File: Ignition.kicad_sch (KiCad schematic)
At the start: 12 parts, among them Q1 AOI21357, Q2 2N7002, Q3 2N7002, Q5 AOI21357

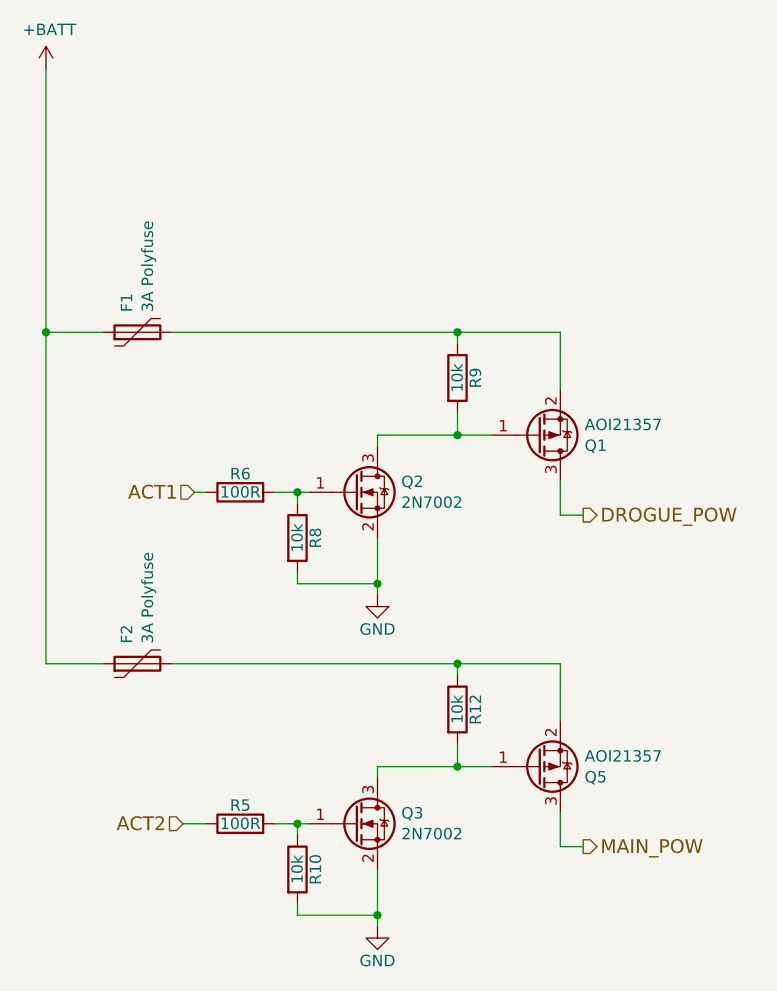
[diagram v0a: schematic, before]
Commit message: fix mosfet
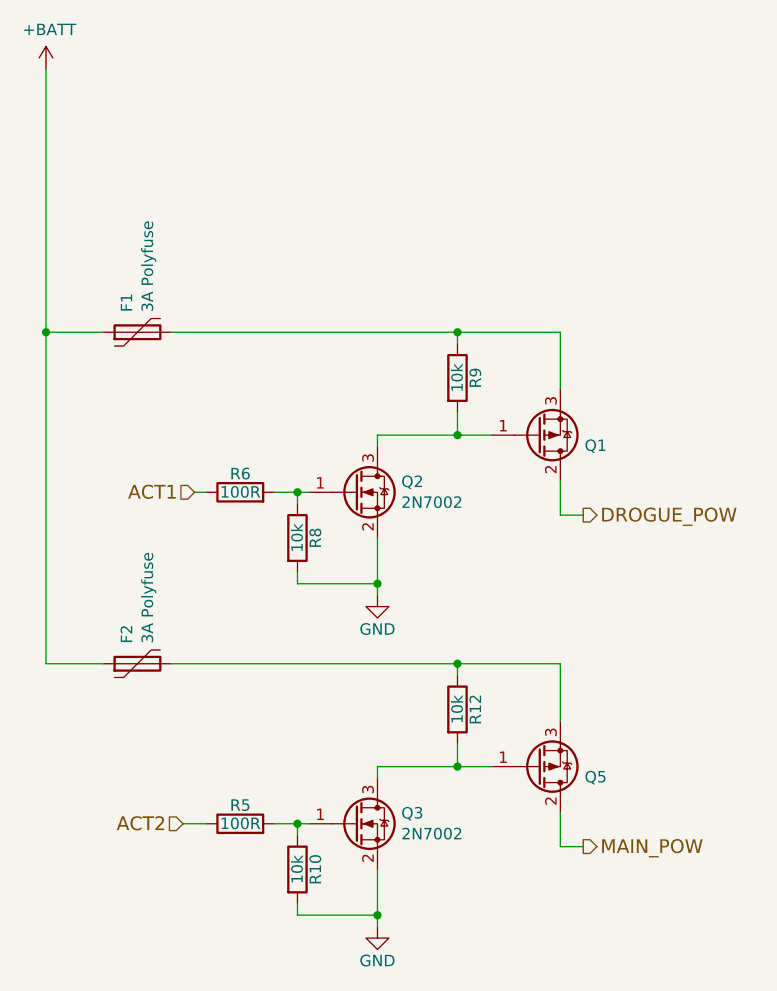
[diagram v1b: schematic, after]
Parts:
- Q1, Q5: value AOI21357 -> (none); footprint Package_TO_SOT_THT:TO-251-3_Vertical -> (none); symbol Device:Q_PMOS_GSD -> Device:Q_PMOS_GDS
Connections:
- net DROGUE_POW: now also Q1.2 (D); no longer Q1.3 (D)
- net MAIN_POW: now also Q5.2 (D); no longer Q5.3 (D)
- net at F1.2, R9.1: now also Q1.3 (S); no longer Q1.2 (S)
- net at F2.2, R12.1: now also Q5.3 (S); no longer Q5.2 (S)
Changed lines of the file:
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@@
+    (stroke (width 0) (type default) (color 0 0 0 0))
+  )
+  (wire (pts (xy 139.7 63.5) (xy 139.7 66.04))
+    (stroke (width 0) (type default) (color 0 0 0 0))
+  )
+  (wire (pts (xy 121.92 110.49) (xy 121.92 109.22))
+    (stroke (width 0) (type default) (color 0 0 0 0))
+  )
+  (wire (pts (xy 130.81 82.55) (xy 130.81 83.82))
+    (stroke (width 0) (type default) (color 0 0 0 0))
+  )
+  (wire (pts (xy 121.92 119.38) (xy 130.81 119.38))
+    (stroke (width 0) (type default) (color 0 0 0 0))
+  )
+  (wire (pts (xy 109.22 109.22) (xy 111.76 109.22))
+    (stroke (width 0) (type default) (color 0 0 0 0))
+  )
+  (wire (pts (xy 139.7 66.04) (xy 143.51 66.04))
+    (stroke (width 0) (type default) (color 0 0 0 0))
+  )
+  (wire (pts (xy 119.38 109.22) (xy 121.92 109.22))
+    (stroke (width 0) (type default) (color 0 0 0 0))
+  )
+  (wire (pts (xy 130.81 66.04) (xy 130.81 67.31))
+    (stroke (width 0) (type default) (color 0 0 0 0))
+  )
+  (wire (pts (xy 139.7 92.71) (xy 139.7 91.44))
+    (stroke (width 0) (type default) (color 0 0 0 0))
+  )
+  (wire (pts (xy 139.7 102.87) (xy 143.51 102.87))
+    (stroke (width 0) (type default) (color 0 0 0 0))
+  )
+  (wire (pts (xy 121.92 81.28) (xy 121.92 82.55))
     (stroke (width 0) (type default) (color 0 0 0 0))
   )
@@
     (stroke (width 0) (type default) (color 0 0 0 0))
   )
-  (wire (pts (xy 139.7 63.5) (xy 139.7 66.04))
-    (stroke (width 0) (type default) (color 0 0 0 0))
-  )
-  (wire (pts (xy 121.92 110.49) (xy 121.92 109.22))
-    (stroke (width 0) (type default) (color 0 0 0 0))
-  )
-  (wire (pts (xy 130.81 82.55) (xy 130.81 83.82))
-    (stroke (width 0) (type default) (color 0 0 0 0))
-  )
-  (wire (pts (xy 121.92 119.38) (xy 130.81 119.38))
-    (stroke (width 0) (type default) (color 0 0 0 0))
-  )
-  (wire (pts (xy 109.22 109.22) (xy 111.76 109.22))
-    (stroke (width 0) (type default) (color 0 0 0 0))
-  )
-  (wire (pts (xy 139.7 66.04) (xy 143.51 66.04))
-    (stroke (width 0) (type default) (color 0 0 0 0))
-  )
-  (wire (pts (xy 119.38 109.22) (xy 121.92 109.22))
-    (stroke (width 0) (type default) (color 0 0 0 0))
-  )
-  (wire (pts (xy 130.81 66.04) (xy 130.81 67.31))
-    (stroke (width 0) (type default) (color 0 0 0 0))
-  )
-  (wire (pts (xy 139.7 92.71) (xy 139.7 91.44))
-    (stroke (width 0) (type default) (color 0 0 0 0))
-  )
-  (wire (pts (xy 139.7 102.87) (xy 143.51 102.87))
-    (stroke (width 0) (type default) (color 0 0 0 0))
-  )
-  (wire (pts (xy 121.92 81.28) (xy 121.92 82.55))
-    (stroke (width 0) (type default) (color 0 0 0 0))
-  )
   (wire (pts (xy 93.98 54.61) (xy 100.33 54.61))
     (stroke (width 0) (type default) (color 0 0 0 0))
@@
     (stroke (width 0) (type default) (color 0 0 0 0))
   )
-  (wire (pts (xy 151.13 74.93) (xy 151.13 71.12))
-    (stroke (width 0) (type default) (color 0 0 0 0))
-  )
   (wire (pts (xy 130.81 102.87) (xy 130.81 104.14))
     (stroke (width 0) (type default) (color 0 0 0 0))
@@
   )
   (wire (pts (xy 130.81 66.04) (xy 139.7 66.04))
+    (stroke (width 0) (type default) (color 0 0 0 0))
+  )
+  (wire (pts (xy 151.13 71.12) (xy 151.13 74.93))
     (stroke (width 0) (type default) (color 0 0 0 0))
   )
@@
     (pin "2")
   )
-  (symbol (lib_id "Device:Q_PMOS_GSD") (at 148.59 102.87 0) (mirror x) (unit 1)
+  (symbol (lib_id "Device:Q_PMOS_GDS") (at 148.59 102.87 0) (mirror x) (unit 1)
     (in_bom yes) (on_board yes)
     (property "Reference" "Q5" (id 0) (at 153.8224 104.0384 0)
       (effects (font (size 1.27 1.27)) (justify left))
     )
-    (property "Value" "AOI21357" (id 1) (at 153.8224 101.727 0)
-      (effects (font (size 1.27 1.27)) (justify left))
-    )
-    (property "Footprint" "Package_TO_SOT_THT:TO-251-3_Vertical" (id 2) (at 153.67 105.41 0)
+    (property "Value" "" (id 1) (at 153.8224 101.727 0)
+      (effects (font (size 1.27 1.27)) (justify left))
+    )
+    (property "Footprint" "" (id 2) (at 153.67 105.41 0)
       (effects (font (size 1.27 1.27)) hide)
     )
@@
     (pin "2")
   )
-  (symbol (lib_id "Device:Q_PMOS_GSD") (at 148.59 66.04 0) (mirror x) (unit 1)
+  (symbol (lib_id "Device:Q_PMOS_GDS") (at 148.59 66.04 0) (mirror x) (unit 1)
     (in_bom yes) (on_board yes)
     (property "Reference" "Q1" (id 0) (at 153.8224 67.2084 0)
       (effects (font (size 1.27 1.27)) (justify left))
     )
-    (property "Value" "AOI21357" (id 1) (at 153.8224 64.897 0)
-      (effects (font (size 1.27 1.27)) (justify left))
-    )
-    (property "Footprint" "Package_TO_SOT_THT:TO-251-3_Vertical" (id 2) (at 153.67 68.58 0)
-      (effects (font (size 1.27 1.27)) hide)
-    )
+    (property "Value" "" (id 1) (at 153.8224 64.897 0)
+      (effects (font (size 1.27 1.27)) (justify left))
+    )
+    (property "Footprint" "" (id 2) (at 153.67 68.58 0)
+      (effects (font (size 1.27 1.27)) hide)
+    )

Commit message: Unmoved parts cause stencil
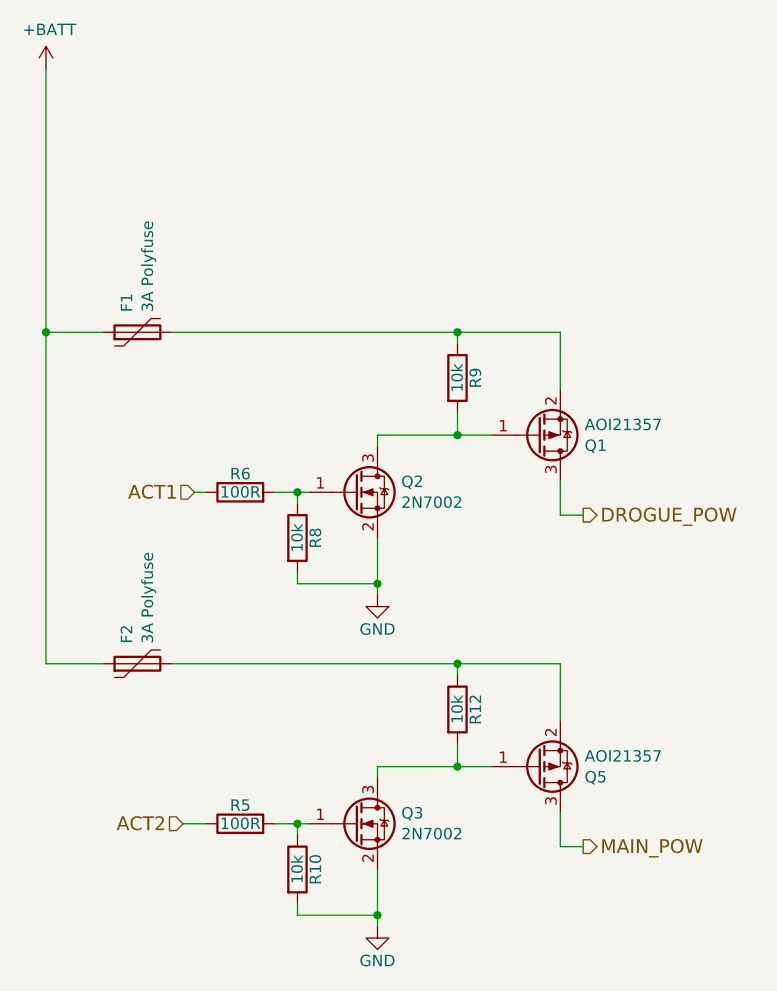
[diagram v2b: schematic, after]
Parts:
- Q1, Q5: value (none) -> AOI21357; footprint (none) -> Package_TO_SOT_THT:TO-251-3_Vertical; symbol Device:Q_PMOS_GDS -> Device:Q_PMOS_GSD
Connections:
- net DROGUE_POW: now also Q1.3 (D); no longer Q1.2 (D)
- net MAIN_POW: now also Q5.3 (D); no longer Q5.2 (D)
- net at F1.2, R9.1: now also Q1.2 (S); no longer Q1.3 (S)
- net at F2.2, R12.1: now also Q5.2 (S); no longer Q5.3 (S)
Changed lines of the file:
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@@
+    (stroke (width 0) (type default) (color 0 0 0 0))
+  )
+  (wire (pts (xy 139.7 54.61) (xy 151.13 54.61))
     (stroke (width 0) (type default) (color 0 0 0 0))
   )
@@
     (stroke (width 0) (type default) (color 0 0 0 0))
   )
-  (wire (pts (xy 139.7 54.61) (xy 151.13 54.61))
-    (stroke (width 0) (type default) (color 0 0 0 0))
-  )
   (wire (pts (xy 93.98 54.61) (xy 100.33 54.61))
     (stroke (width 0) (type default) (color 0 0 0 0))
@@
     (stroke (width 0) (type default) (color 0 0 0 0))
   )
+  (wire (pts (xy 151.13 74.93) (xy 151.13 71.12))
+    (stroke (width 0) (type default) (color 0 0 0 0))
+  )
   (wire (pts (xy 130.81 102.87) (xy 130.81 104.14))
     (stroke (width 0) (type default) (color 0 0 0 0))
@@
   )
   (wire (pts (xy 130.81 66.04) (xy 139.7 66.04))
-    (stroke (width 0) (type default) (color 0 0 0 0))
-  )
-  (wire (pts (xy 151.13 71.12) (xy 151.13 74.93))
     (stroke (width 0) (type default) (color 0 0 0 0))
   )
@@
     (pin "2")
   )
-  (symbol (lib_id "Device:Q_PMOS_GDS") (at 148.59 102.87 0) (mirror x) (unit 1)
+  (symbol (lib_id "Device:Q_PMOS_GSD") (at 148.59 102.87 0) (mirror x) (unit 1)
     (in_bom yes) (on_board yes)
     (property "Reference" "Q5" (id 0) (at 153.8224 104.0384 0)
       (effects (font (size 1.27 1.27)) (justify left))
     )
-    (property "Value" "" (id 1) (at 153.8224 101.727 0)
-      (effects (font (size 1.27 1.27)) (justify left))
-    )
-    (property "Footprint" "" (id 2) (at 153.67 105.41 0)
+    (property "Value" "AOI21357" (id 1) (at 153.8224 101.727 0)
+      (effects (font (size 1.27 1.27)) (justify left))
+    )
+    (property "Footprint" "Package_TO_SOT_THT:TO-251-3_Vertical" (id 2) (at 153.67 105.41 0)
       (effects (font (size 1.27 1.27)) hide)
     )
@@
     (pin "2")
   )
-  (symbol (lib_id "Device:Q_PMOS_GDS") (at 148.59 66.04 0) (mirror x) (unit 1)
+  (symbol (lib_id "Device:Q_PMOS_GSD") (at 148.59 66.04 0) (mirror x) (unit 1)
     (in_bom yes) (on_board yes)
     (property "Reference" "Q1" (id 0) (at 153.8224 67.2084 0)
       (effects (font (size 1.27 1.27)) (justify left))
     )
-    (property "Value" "" (id 1) (at 153.8224 64.897 0)
-      (effects (font (size 1.27 1.27)) (justify left))
-    )
-    (property "Footprint" "" (id 2) (at 153.67 68.58 0)
-      (effects (font (size 1.27 1.27)) hide)
-    )
+    (property "Value" "AOI21357" (id 1) (at 153.8224 64.897 0)
+      (effects (font (size 1.27 1.27)) (justify left))
+    )
+    (property "Footprint" "Package_TO_SOT_THT:TO-251-3_Vertical" (id 2) (at 153.67 68.58 0)
+      (effects (font (size 1.27 1.27)) hide)
+    )
